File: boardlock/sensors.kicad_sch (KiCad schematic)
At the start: 31 parts, among them Q2 MMBT4401, Q4 BSS84PWH6327XTSA1, U1 LSM6DSO32, U3 SAM-M8Q

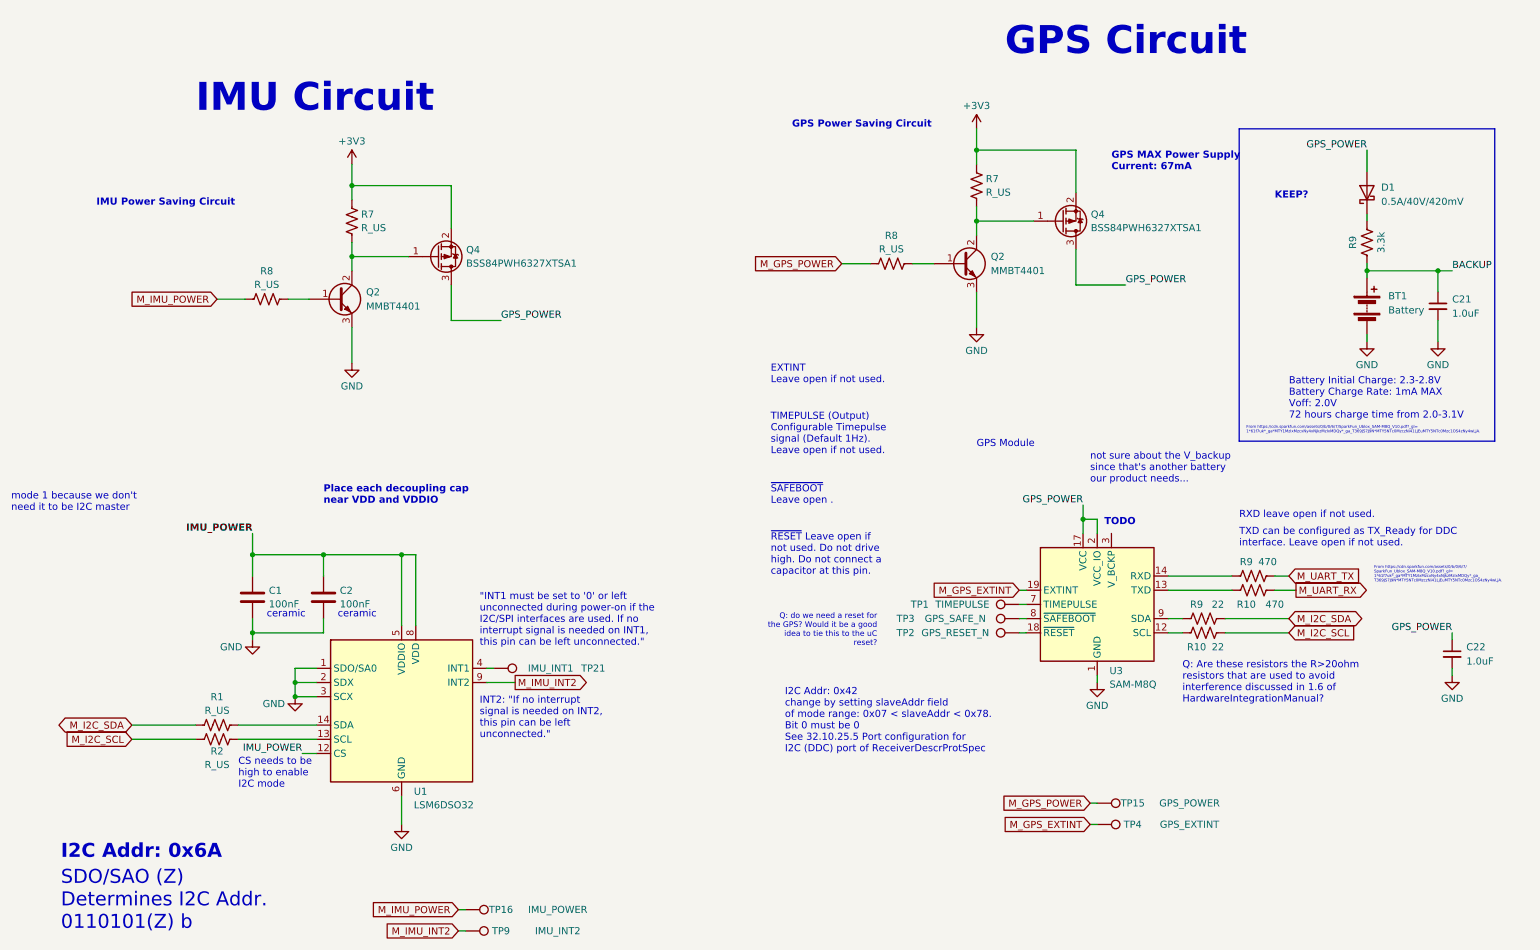
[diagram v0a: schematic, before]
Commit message: more Zecong edits
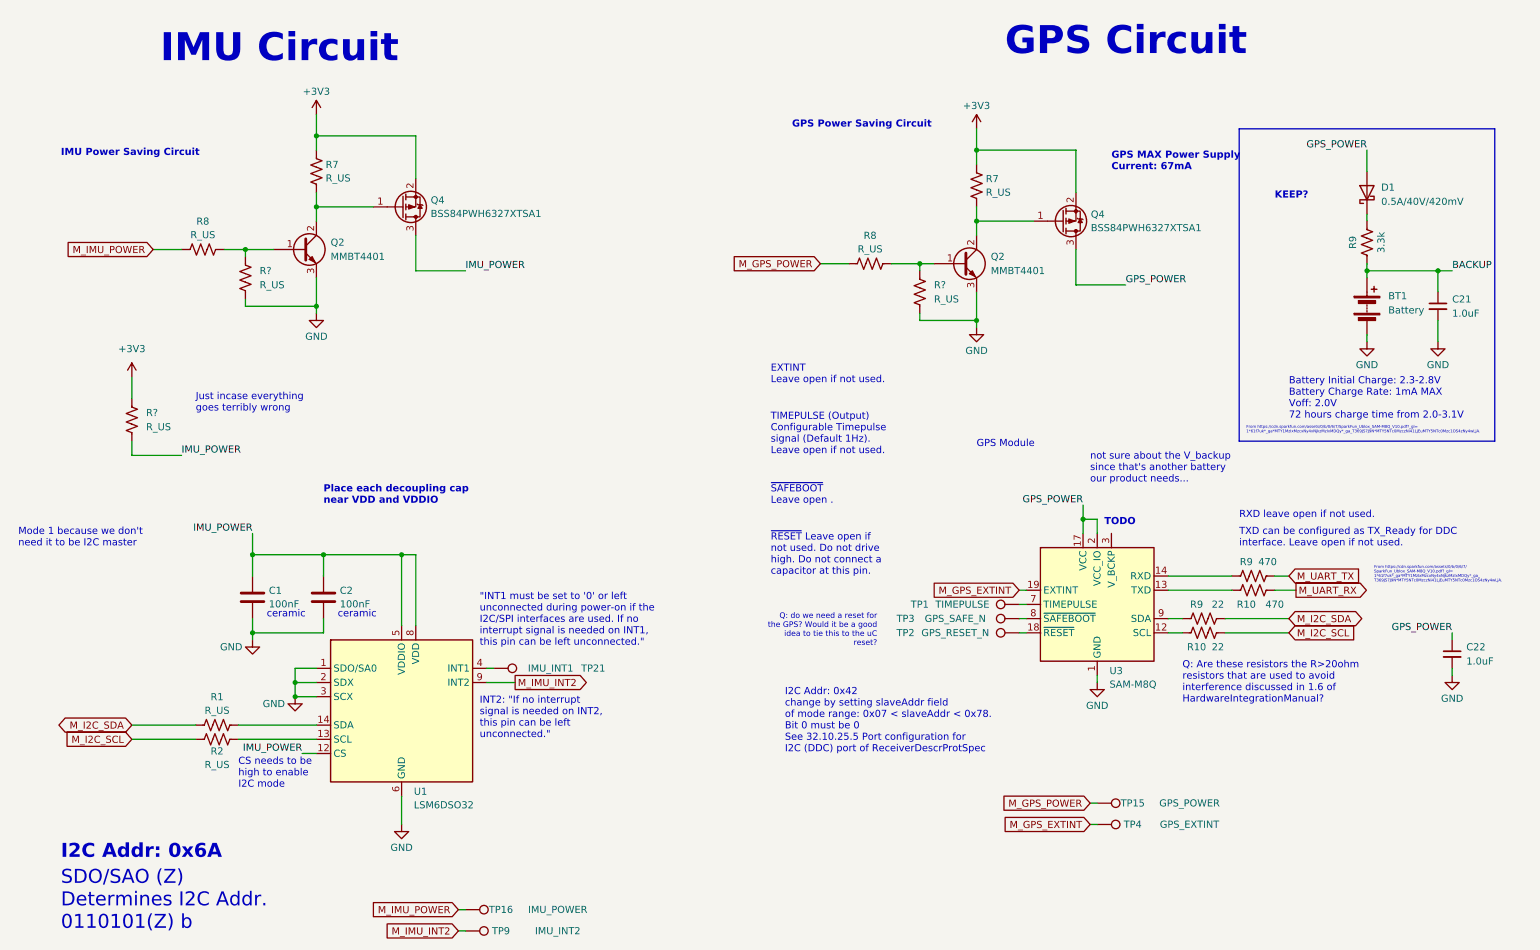
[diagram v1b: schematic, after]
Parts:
- added R? (x3): R_US, symbol Device:R_US
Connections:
- net +3V3: now also R?.1
- net GND: now also R?.2, R?.2
- net GPS_POWER: no longer Q4.3 (D)
- net IMU_POWER: now also Q4.3 (D), R?.2
- net at Q2.1 (B), R8.2: now also R?.1 (x2)
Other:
- note added: "Just incase everything goes terribly wrong"
- note added: "Mode 1 because we don't need it to be I2C master"
- note removed: "mode 1 because we don't need it to be I2C master"
- moved on the sheet: Q2, Q4, R7, R8
